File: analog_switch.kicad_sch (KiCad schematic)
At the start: 8 parts, among them U1 ADG1607xCP, U2 ADG1607xCP, U3 ADG1607xCP, U4 ADG1607xCP, U5 ADG1607xCP, U6 ADG1607xCP, U7 ADG1607xCP, U8 ADG1607xCP

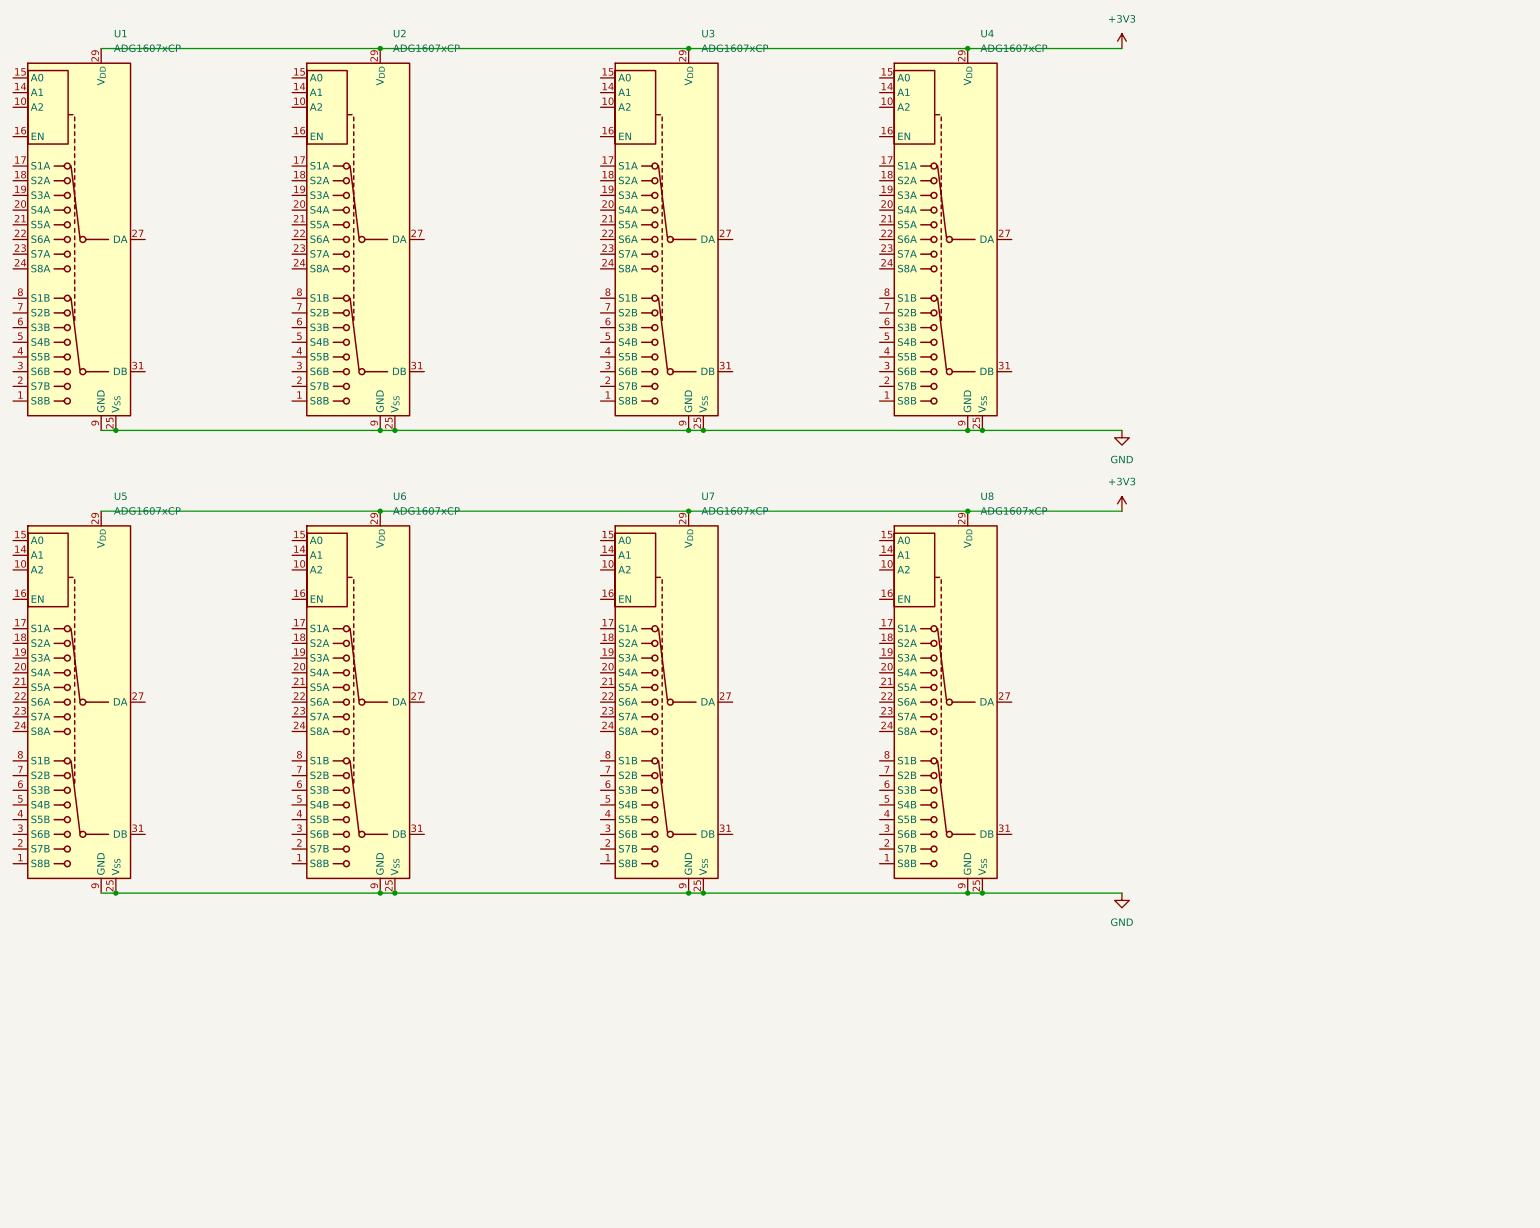
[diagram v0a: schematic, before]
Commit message: sch
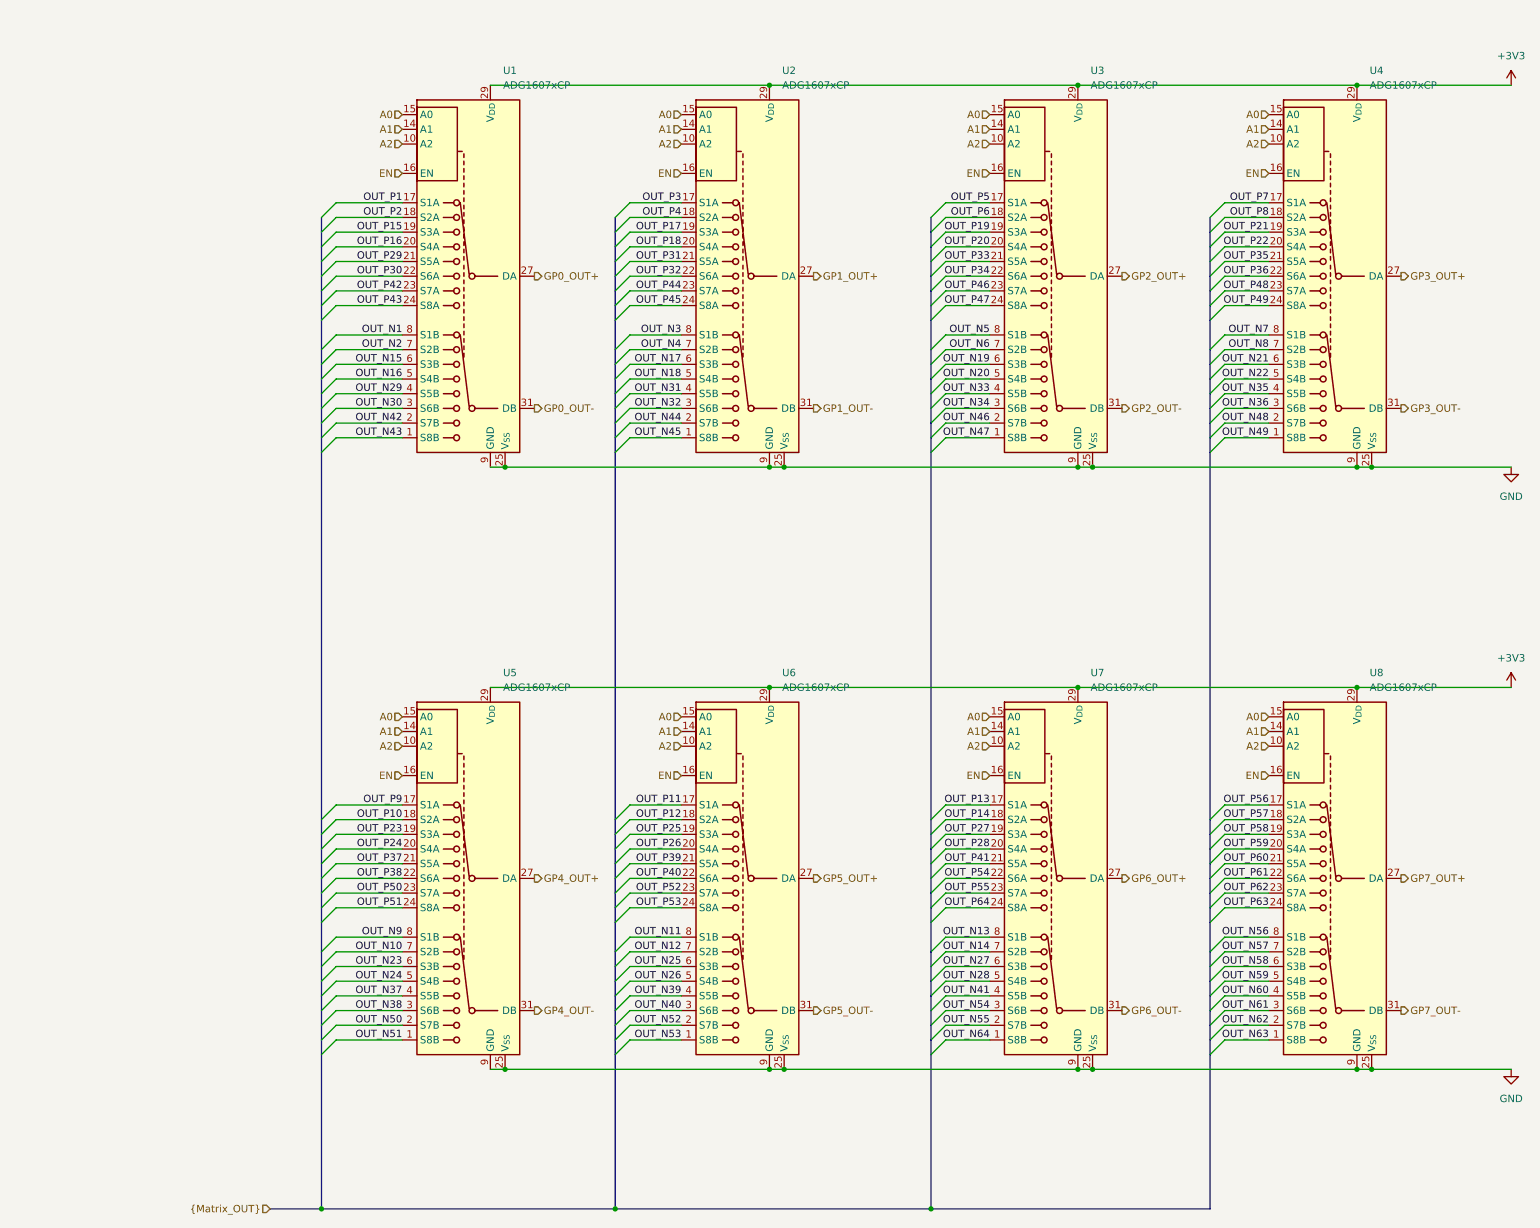
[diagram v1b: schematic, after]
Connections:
- net OUT_N43: now reaches U1.1 (S8B)
- net A2: now reaches U1.10 (A2)
- net A2: now also U2.10 (A2), U3.10 (A2), U4.10 (A2), U5.10 (A2), U6.10 (A2), U7.10 (A2), U8.10 (A2)
- net A1: now reaches U1.14 (A1)
- net A1: now also U2.14 (A1), U3.14 (A1), U4.14 (A1), U5.14 (A1), U6.14 (A1), U7.14 (A1), U8.14 (A1)
- net A0: now reaches U1.15 (A0)
- net A0: now also U2.15 (A0), U3.15 (A0), U4.15 (A0), U5.15 (A0), U6.15 (A0), U7.15 (A0), U8.15 (A0)
- net EN: now reaches U1.16 (EN)
- net EN: now also U2.16 (EN), U3.16 (EN), U4.16 (EN), U5.16 (EN), U6.16 (EN), U7.16 (EN), U8.16 (EN)
- net OUT_P1: now reaches U1.17 (S1A)
- net OUT_P2: now reaches U1.18 (S2A)
- net OUT_P15: now reaches U1.19 (S3A)
- net OUT_N42: now reaches U1.2 (S7B)
- net OUT_P16: now reaches U1.20 (S4A)
- net OUT_P29: now reaches U1.21 (S5A)
- net OUT_P30: now reaches U1.22 (S6A)
- net OUT_P42: now reaches U1.23 (S7A)
- net OUT_P43: now reaches U1.24 (S8A)
- net GP0_OUT+: now reaches U1.27 (DA)
- net OUT_N30: now reaches U1.3 (S6B)
- net GP0_OUT-: now reaches U1.31 (DB)
- net OUT_N29: now reaches U1.4 (S5B)
- net OUT_N16: now reaches U1.5 (S4B)
- net OUT_N15: now reaches U1.6 (S3B)
- net OUT_N2: now reaches U1.7 (S2B)
- net OUT_N1: now reaches U1.8 (S1B)
- net OUT_N45: now reaches U2.1 (S8B)
- net OUT_P3: now reaches U2.17 (S1A)
- net OUT_P4: now reaches U2.18 (S2A)
- net OUT_P17: now reaches U2.19 (S3A)
- net OUT_N44: now reaches U2.2 (S7B)
- net OUT_P18: now reaches U2.20 (S4A)
- net OUT_P31: now reaches U2.21 (S5A)
- net OUT_P32: now reaches U2.22 (S6A)
- net OUT_P44: now reaches U2.23 (S7A)
- net OUT_P45: now reaches U2.24 (S8A)
- net GP1_OUT+: now reaches U2.27 (DA)
- net OUT_N32: now reaches U2.3 (S6B)
- net GP1_OUT-: now reaches U2.31 (DB)
- net OUT_N31: now reaches U2.4 (S5B)
- net OUT_N18: now reaches U2.5 (S4B)
- net OUT_N17: now reaches U2.6 (S3B)
- net OUT_N4: now reaches U2.7 (S2B)
- net OUT_N3: now reaches U2.8 (S1B)
- net OUT_N53: now reaches U6.1 (S8B)
- net OUT_P11: now reaches U6.17 (S1A)
- net OUT_P12: now reaches U6.18 (S2A)
- net OUT_P25: now reaches U6.19 (S3A)
- net OUT_N52: now reaches U6.2 (S7B)
- net OUT_P26: now reaches U6.20 (S4A)
- net OUT_P39: now reaches U6.21 (S5A)
- net OUT_P40: now reaches U6.22 (S6A)
- net OUT_P52: now reaches U6.23 (S7A)
- net OUT_P53: now reaches U6.24 (S8A)
- net GP5_OUT+: now reaches U6.27 (DA)
- net OUT_N40: now reaches U6.3 (S6B)
- net GP5_OUT-: now reaches U6.31 (DB)
- net OUT_N39: now reaches U6.4 (S5B)
- net OUT_N26: now reaches U6.5 (S4B)
- net OUT_N25: now reaches U6.6 (S3B)
- net OUT_N12: now reaches U6.7 (S2B)
- net OUT_N11: now reaches U6.8 (S1B)
- net OUT_N63: now reaches U8.1 (S8B)
- net OUT_P56: now reaches U8.17 (S1A)
- net OUT_P57: now reaches U8.18 (S2A)
- net OUT_P58: now reaches U8.19 (S3A)
- net OUT_N62: now reaches U8.2 (S7B)
- net OUT_P59: now reaches U8.20 (S4A)
- net OUT_P60: now reaches U8.21 (S5A)
- net OUT_P61: now reaches U8.22 (S6A)
- net OUT_P62: now reaches U8.23 (S7A)
- net OUT_P63: now reaches U8.24 (S8A)
- net GP7_OUT+: now reaches U8.27 (DA)
- net OUT_N61: now reaches U8.3 (S6B)
- net GP7_OUT-: now reaches U8.31 (DB)
- net OUT_N60: now reaches U8.4 (S5B)
- net OUT_N59: now reaches U8.5 (S4B)
- net OUT_N58: now reaches U8.6 (S3B)
- net OUT_N57: now reaches U8.7 (S2B)
- net OUT_N56: now reaches U8.8 (S1B)
- net OUT_N49: now reaches U4.1 (S8B)
- net OUT_P7: now reaches U4.17 (S1A)
- net OUT_P8: now reaches U4.18 (S2A)
- net OUT_P21: now reaches U4.19 (S3A)
- net OUT_N48: now reaches U4.2 (S7B)
- net OUT_P22: now reaches U4.20 (S4A)
- net OUT_P35: now reaches U4.21 (S5A)
- net OUT_P36: now reaches U4.22 (S6A)
- net OUT_P48: now reaches U4.23 (S7A)
- net OUT_P49: now reaches U4.24 (S8A)
- net GP3_OUT+: now reaches U4.27 (DA)
- net OUT_N36: now reaches U4.3 (S6B)
- net GP3_OUT-: now reaches U4.31 (DB)
- net OUT_N35: now reaches U4.4 (S5B)
- net OUT_N22: now reaches U4.5 (S4B)
- net OUT_N21: now reaches U4.6 (S3B)
- net OUT_N8: now reaches U4.7 (S2B)
- net OUT_N7: now reaches U4.8 (S1B)
- net OUT_N64: now reaches U7.1 (S8B)
- net OUT_P13: now reaches U7.17 (S1A)
- net OUT_P14: now reaches U7.18 (S2A)
- net OUT_P27: now reaches U7.19 (S3A)
- net OUT_N55: now reaches U7.2 (S7B)
- net OUT_P28: now reaches U7.20 (S4A)
- net OUT_P41: now reaches U7.21 (S5A)
- net OUT_P54: now reaches U7.22 (S6A)
- net OUT_P55: now reaches U7.23 (S7A)
- net OUT_P64: now reaches U7.24 (S8A)
- net GP6_OUT+: now reaches U7.27 (DA)
- net OUT_N54: now reaches U7.3 (S6B)
- net GP6_OUT-: now reaches U7.31 (DB)
- net OUT_N41: now reaches U7.4 (S5B)
- net OUT_N28: now reaches U7.5 (S4B)
- net OUT_N27: now reaches U7.6 (S3B)
- net OUT_N14: now reaches U7.7 (S2B)
- net OUT_N13: now reaches U7.8 (S1B)
- net OUT_N47: now reaches U3.1 (S8B)
- net OUT_P5: now reaches U3.17 (S1A)
- net OUT_P6: now reaches U3.18 (S2A)
- net OUT_P19: now reaches U3.19 (S3A)
- net OUT_N46: now reaches U3.2 (S7B)
- net OUT_P20: now reaches U3.20 (S4A)
- net OUT_P33: now reaches U3.21 (S5A)
- net OUT_P34: now reaches U3.22 (S6A)
- net OUT_P46: now reaches U3.23 (S7A)
- net OUT_P47: now reaches U3.24 (S8A)
- net GP2_OUT+: now reaches U3.27 (DA)
- net OUT_N34: now reaches U3.3 (S6B)
- net GP2_OUT-: now reaches U3.31 (DB)
- net OUT_N33: now reaches U3.4 (S5B)
- net OUT_N20: now reaches U3.5 (S4B)
- net OUT_N19: now reaches U3.6 (S3B)
- net OUT_N6: now reaches U3.7 (S2B)
- net OUT_N5: now reaches U3.8 (S1B)
- net OUT_N51: now reaches U5.1 (S8B)
- net OUT_P9: now reaches U5.17 (S1A)
- net OUT_P10: now reaches U5.18 (S2A)
- net OUT_P23: now reaches U5.19 (S3A)
- net OUT_N50: now reaches U5.2 (S7B)
- net OUT_P24: now reaches U5.20 (S4A)
- net OUT_P37: now reaches U5.21 (S5A)
- net OUT_P38: now reaches U5.22 (S6A)
- net OUT_P50: now reaches U5.23 (S7A)
- net OUT_P51: now reaches U5.24 (S8A)
- net GP4_OUT+: now reaches U5.27 (DA)
- net OUT_N38: now reaches U5.3 (S6B)
- net GP4_OUT-: now reaches U5.31 (DB)
- net OUT_N37: now reaches U5.4 (S5B)
- net OUT_N24: now reaches U5.5 (S4B)
- net OUT_N23: now reaches U5.6 (S3B)
- net OUT_N10: now reaches U5.7 (S2B)
- net OUT_N9: now reaches U5.8 (S1B)
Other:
- moved on the sheet: U1, U2, U3, U4, U5, U6, U7, U8
